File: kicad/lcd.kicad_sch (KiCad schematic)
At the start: 7 parts, among them J7 R61529 LCD, J8 FT6236, Q5 DMN2004WK-7

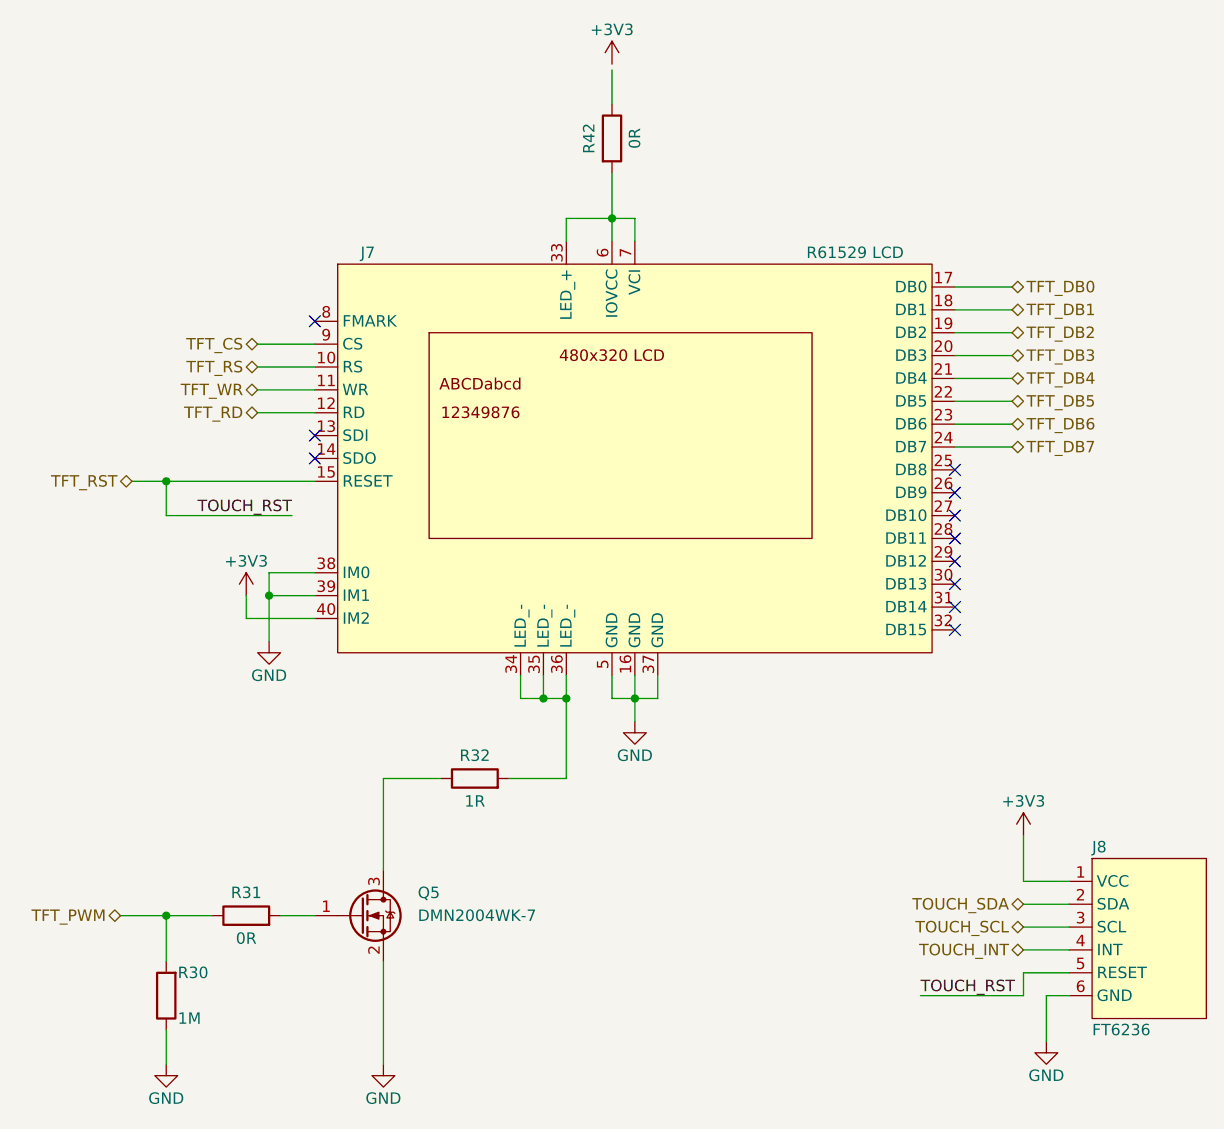
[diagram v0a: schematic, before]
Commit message: add rules to .gitignore
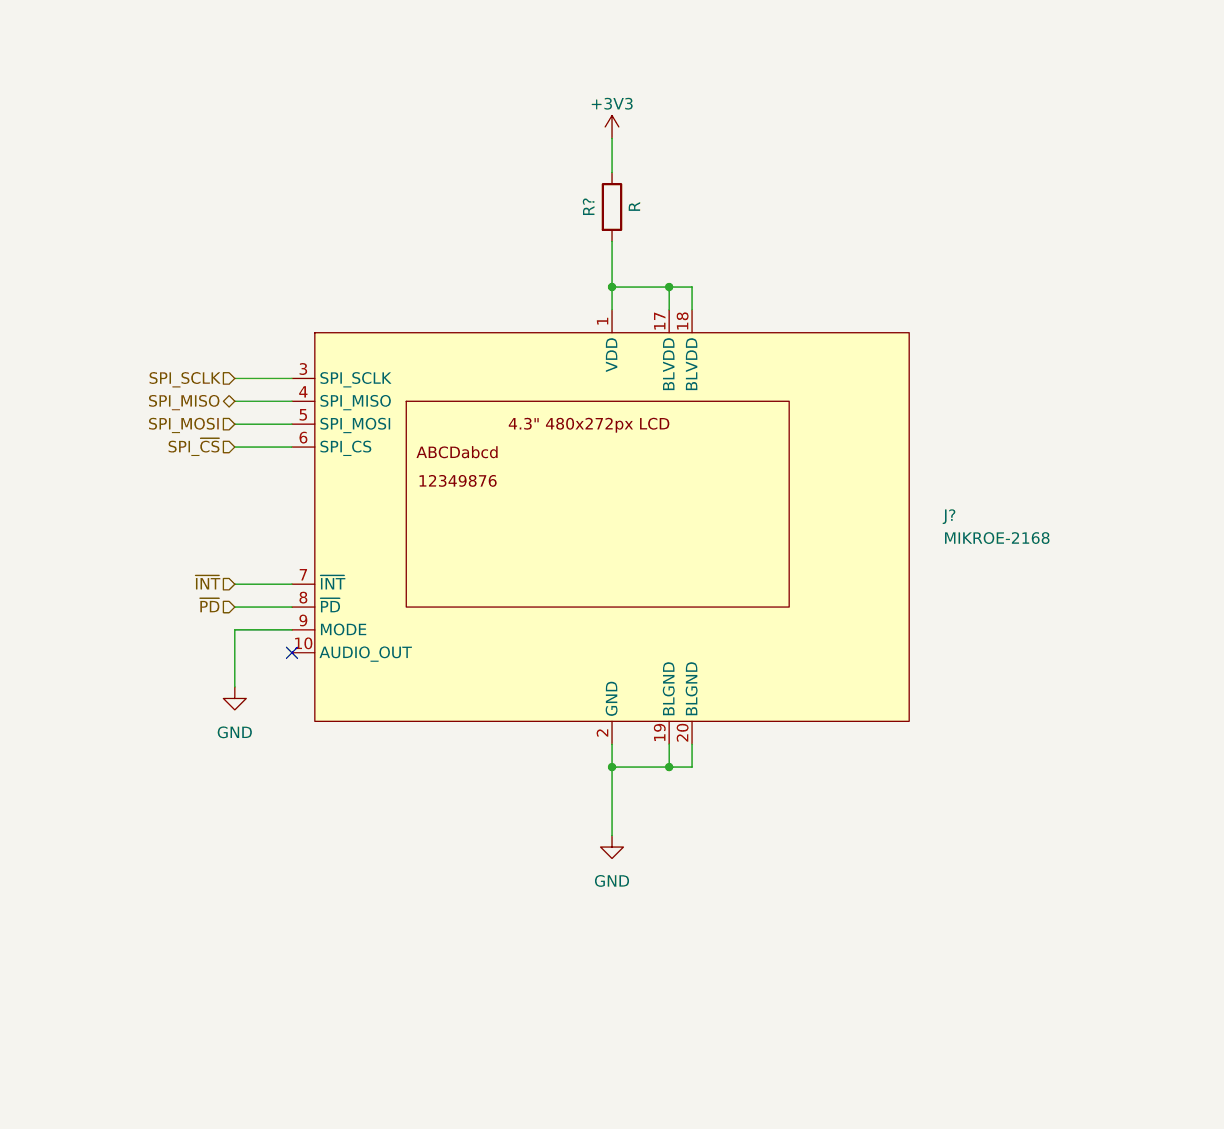
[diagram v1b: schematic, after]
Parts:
- removed J7: R61529 LCD, z_connector:62684-402100ALF, symbol z_ic:R61529 LCD
- removed J8: FT6236, z_connector:SFV6R-2STE1HLF, symbol z_ic:FT6236
- removed Q5: DMN2004WK-7, Package_TO_SOT_SMD:SOT-323_SC-70, symbol z_ic:DMN2004WK-7
- removed R30: 1M, Resistor_SMD:R_0603_1608Metric, symbol Device:R
- removed R31: 0R, Resistor_SMD:R_0603_1608Metric, symbol Device:R
- removed R32: 1R, Resistor_SMD:R_1206_3216Metric, symbol Device:R
- added J?: MIKROE-2168, z_connector:FPC_BOTTOM_20POS_Würth_68712014522, symbol z_ic:MIKROE-2168
- R?: renamed from R42; value 0R -> R
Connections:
- net +3V3: now also R?.1
- net GND: now also J?.19 (BLGND), J?.2 (GND), J?.20 (BLGND), J?.9 (MODE)
- net at R?.2: now also J?.1 (VDD), J?.17 (BLVDD), J?.18 (BLVDD)
- new net: J?.11, J?.12, J?.13, J?.14, J?.15, J?.16
- new net SPI_MISO: J?.4 (SPI_MISO)
- new net SPI_MOSI: J?.5 (SPI_MOSI)
- new net SPI_SCLK: J?.3 (SPI_SCLK)
- new net SPI_~{CS}: J?.6 (SPI_CS)
- new net ~{INT}: J?.7 (~{INT})
- new net ~{PD}: J?.8 (~{PD})
- no-connect marks 11 -> 1
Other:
- moved on the sheet: R?
